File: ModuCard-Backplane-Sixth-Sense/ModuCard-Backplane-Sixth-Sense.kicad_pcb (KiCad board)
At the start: 2 copper layers, 90 parts, among them J16 09031967921, J17 09031967921, J18 09031967921, J19 09031967921, J2 09031967921, J20 09031967921, J21 09031967921, J4 09031967921, SW1 SW_DIP_x02, SW2 SW_DIP_x02, U3 AMS1117, U4 FE2.1, U801 FSUSB42UMX, U802 FSUSB42UMX, X2 X322512MSB4SI

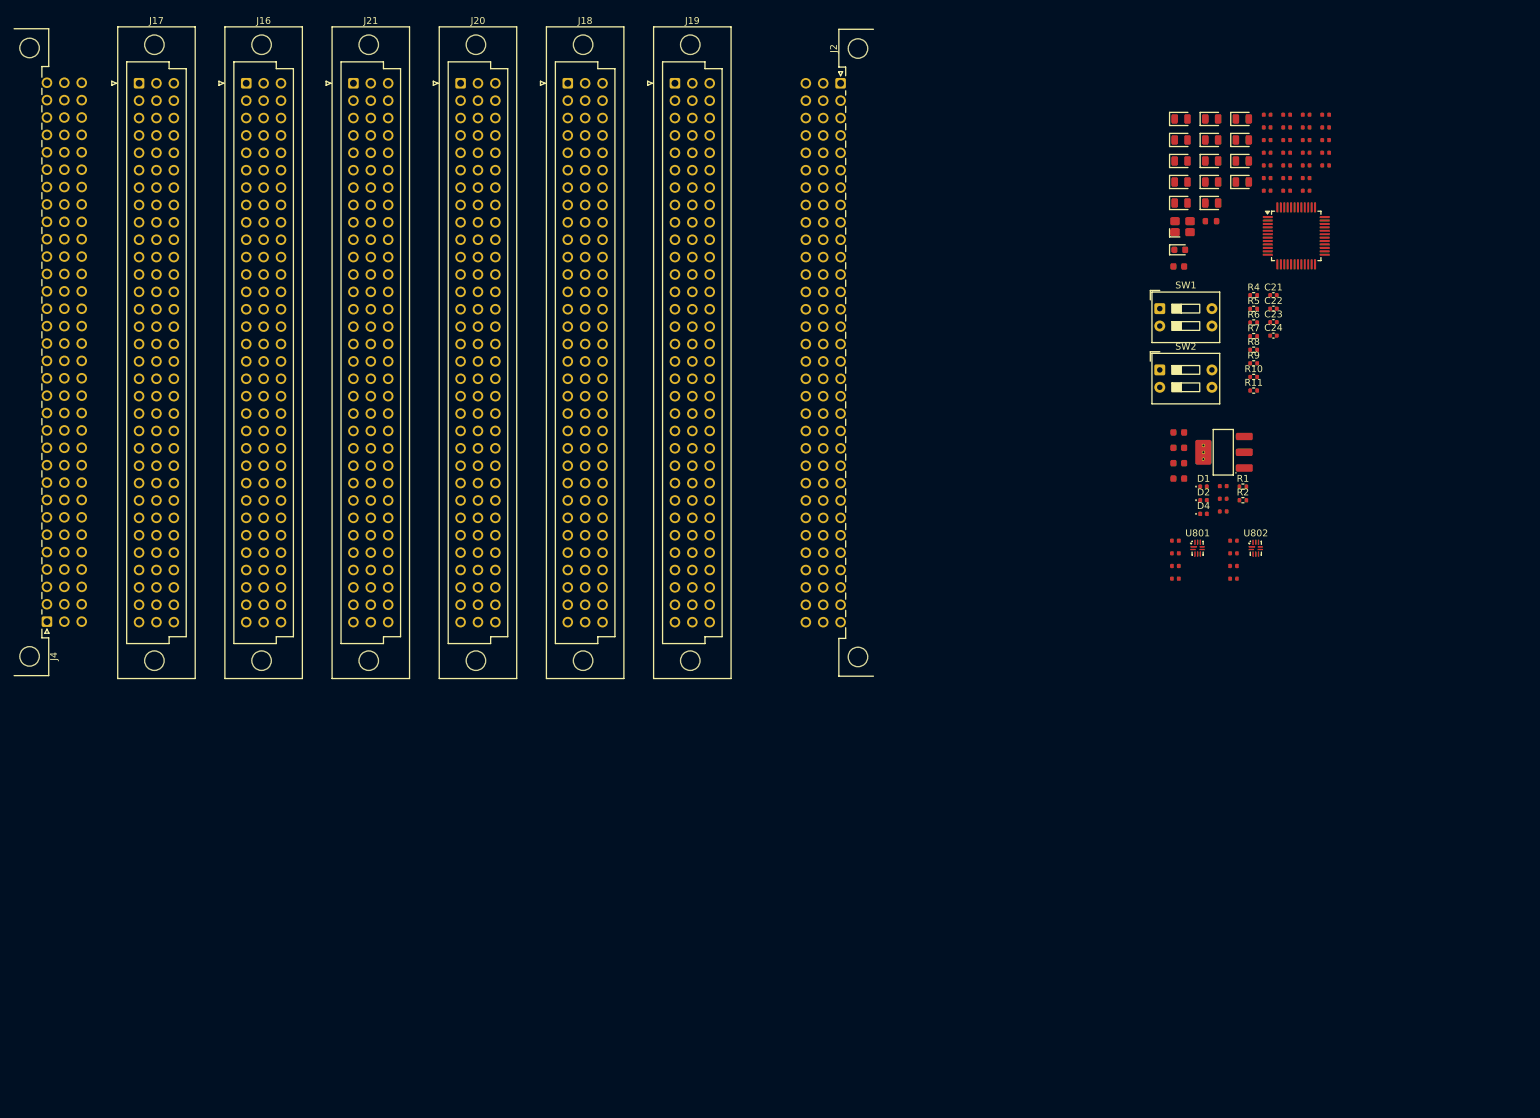
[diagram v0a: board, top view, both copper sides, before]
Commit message: erc -fix1
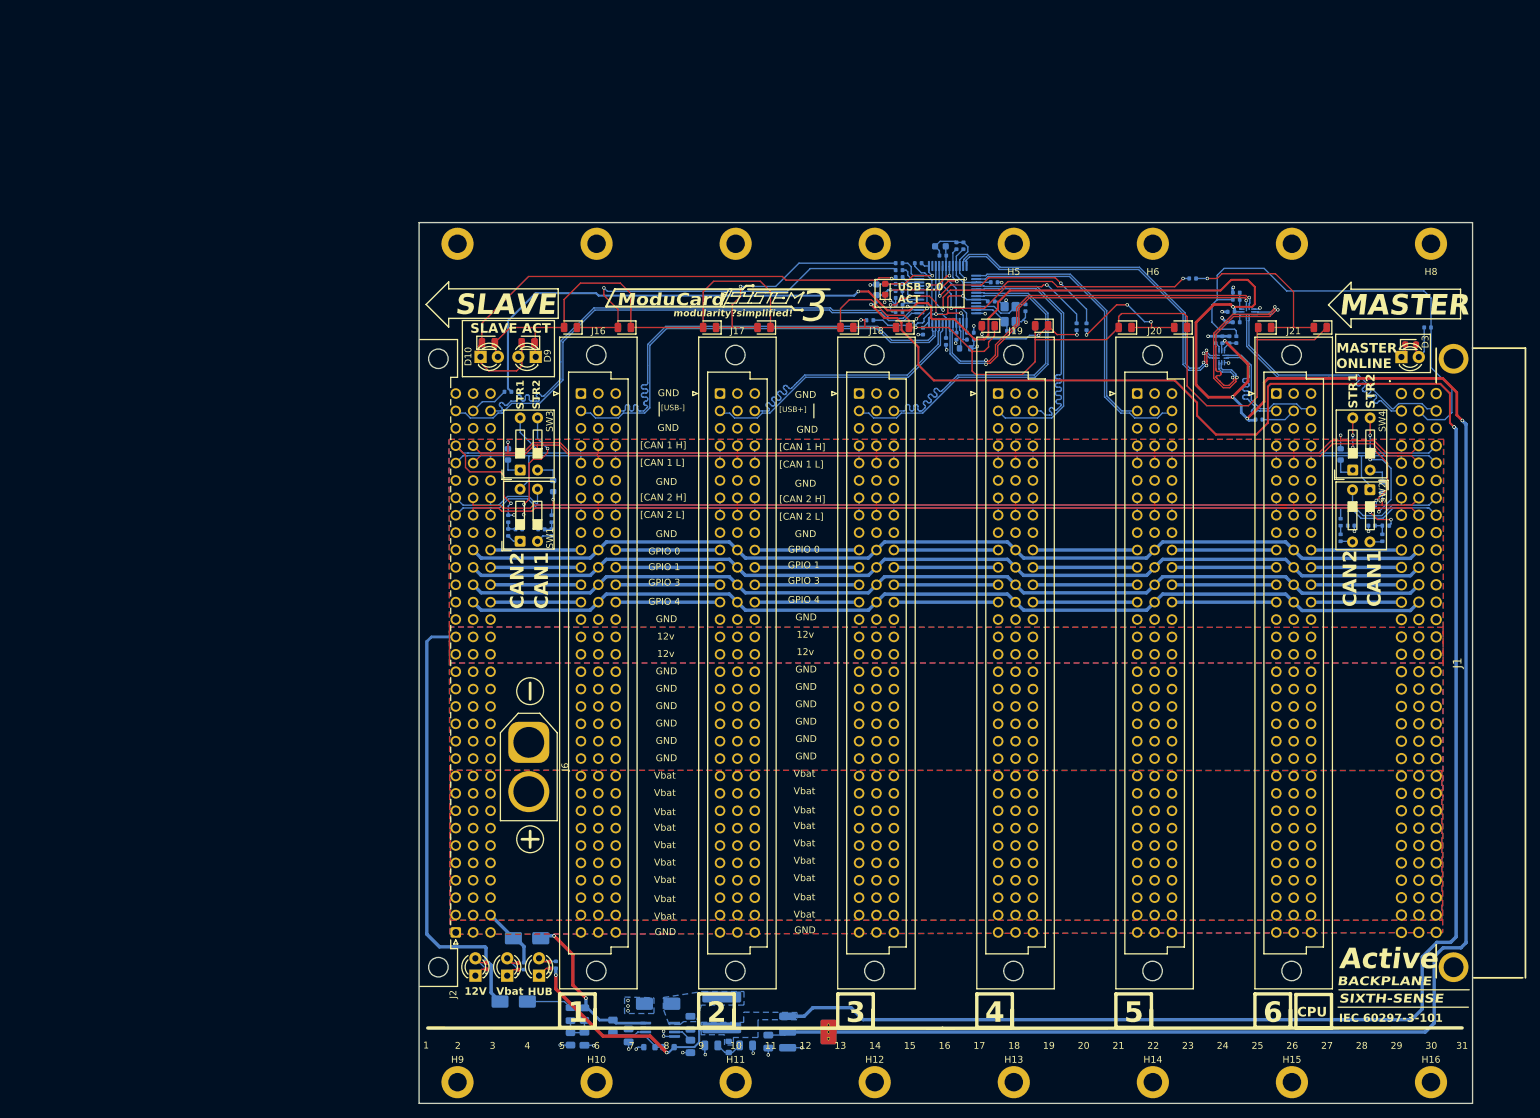
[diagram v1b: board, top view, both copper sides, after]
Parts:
- removed C28: 100nF, PCM_JLCPCB:C_0402
- removed C3, C5: 10uF, PCM_JLCPCB:C_0603
- removed C4, C6: 100nF, PCM_JLCPCB:C_0603
- removed J4: 09031967921, Connector_DIN:DIN41612_R_3x32_Female_Horizontal_THT
- removed R2: 1K2, Resistor_SMD:R_0402_1005Metric
- added C1: 10nF, PCM_JLCPCB:C_0805, B.Cu at (173.2, 200.7)
- added C10: 10uF, PCM_JLCPCB:C_0805, B.Cu at (176.3, 204.0)
- added C11: 10uF, PCM_JLCPCB:C_0805, B.Cu at (184.6, 203.4)
- added C2: 100nF, PCM_JLCPCB:C_0805, B.Cu at (164.2, 202.5)
- added C41: 10uF, PCM_JLCPCB:C_0603, B.Cu at (200.4, 93.5)
- added C7: 10uF, PCM_JLCPCB:C_0805, B.Cu at (155.7, 199.4)
- added C8: 10uF, PCM_JLCPCB:C_0805, B.Cu at (157.7, 203.0)
- added C9: 10uF, PCM_JLCPCB:C_0805, B.Cu at (181.4, 204.0)
- added D10: LED, LED_THT:LED_D3.0mm, F.Cu at (142.6, 103.3)
- added D11: LED, LED_THT:LED_D3.0mm, F.Cu at (141.8, 193.8)
- added D12: LED, LED_THT:LED_D3.0mm, F.Cu at (146.4, 193.8)
- added D13: LED, LED_THT:LED_D3.0mm, F.Cu at (151.1, 193.8)
- added D3: LED, LED_THT:LED_D3.0mm_Clear, F.Cu at (277.1, 103.4)
- added D5: SS510, PCM_JLCPCB:D_SMA, B.Cu at (168.5, 197.9)
- added D6: SS510, PCM_JLCPCB:D_SMA, B.Cu at (149.3, 188.3)
- added D7: SS510, PCM_JLCPCB:D_SMA, B.Cu at (147.4, 197.6)
- added D8: RED, Diode_SMD:D_0402_1005Metric, F.Cu at (152.7, 192.2)
- added D9: LED, LED_THT:LED_D3.0mm, F.Cu at (150.6, 103.3)
- added G***: LOGO, LOGO, B.Cu at (264.6, 200.7)
- added G***: LOGO, LOGO, B.Cu at (246.2, 200.5)
- added H1: MountingHole, MountingHole:MountingHole_2.7mm_M2.5_DIN965_Pad, F.Cu at (139.2, 86.8)
- added H10: MountingHole, MountingHole:MountingHole_2.7mm_M2.5_DIN965_Pad, F.Cu at (159.5, 209.3)
- added H11: MountingHole, MountingHole:MountingHole_2.7mm_M2.5_DIN965_Pad, F.Cu at (179.8, 209.3)
- added H12: MountingHole, MountingHole:MountingHole_2.7mm_M2.5_DIN965_Pad, F.Cu at (200.1, 209.3)
- added H13: MountingHole, MountingHole:MountingHole_2.7mm_M2.5_DIN965_Pad, F.Cu at (220.5, 209.3)
- added H14: MountingHole, MountingHole:MountingHole_2.7mm_M2.5_DIN965_Pad, F.Cu at (240.8, 209.3)
- added H15: MountingHole, MountingHole:MountingHole_2.7mm_M2.5_DIN965_Pad, F.Cu at (261.1, 209.3)
- added H16: MountingHole, MountingHole:MountingHole_2.7mm_M2.5_DIN965_Pad, F.Cu at (281.4, 209.3)
- added H2: MountingHole, MountingHole:MountingHole_2.7mm_M2.5_DIN965_Pad, F.Cu at (159.5, 86.8)
- added H3: MountingHole, MountingHole:MountingHole_2.7mm_M2.5_DIN965_Pad, F.Cu at (179.8, 86.8)
- added H4: MountingHole, MountingHole:MountingHole_2.7mm_M2.5_DIN965_Pad, F.Cu at (200.1, 86.8)
- added H5: MountingHole, MountingHole:MountingHole_2.7mm_M2.5_DIN965_Pad, F.Cu at (220.5, 86.8)
- added H6: MountingHole, MountingHole:MountingHole_2.7mm_M2.5_DIN965_Pad, F.Cu at (240.8, 86.8)
- added H7: MountingHole, MountingHole:MountingHole_2.7mm_M2.5_DIN965_Pad, F.Cu at (261.1, 86.8)
- added H8: MountingHole, MountingHole:MountingHole_2.7mm_M2.5_DIN965_Pad, F.Cu at (281.4, 86.8)
- added H9: MountingHole, MountingHole:MountingHole_2.7mm_M2.5_DIN965_Pad, F.Cu at (139.2, 209.3)
- added J1: 09031967921, Din:09031967921, F.Cu at (282.2, 108.7)
- added J6: Conn_01x02_Pin, Connector_AMASS:AMASS_XT60-F_1x02_P7.20mm_Vertical, F.Cu at (149.6, 159.7)
- added L1: FNR6045S101MT 100uH, Inductor_SMD:L_Chilisin_BWVS00606020, B.Cu at (177.8, 199.1)
- added R12: 100kΩ, PCM_JLCPCB:R_0805, B.Cu at (173.2, 204.1)
- added R13: 3kΩ, PCM_JLCPCB:R_0603, B.Cu at (170.0, 204.2)
- added R14: 3kΩ, PCM_JLCPCB:R_0603, B.Cu at (167.2, 204.2)
- added R15: 100kΩ, PCM_JLCPCB:R_0805, B.Cu at (157.7, 199.4)
- added R16: 100kΩ, PCM_JLCPCB:R_0805, B.Cu at (155.7, 203.0)
- added R17: 1Ω, PCM_JLCPCB:R_0603, B.Cu at (178.8, 204.2)
- added R18: 1K2, Resistor_SMD:R_0402_1005Metric, B.Cu at (153.6, 192.2)
- added R21: 100Ω, PCM_JLCPCB:R_0603, B.Cu at (146.6, 117.6)
- added R22: 100Ω, PCM_JLCPCB:R_0603, B.Cu at (153.2, 122.2)
- added R23: 100Ω, PCM_JLCPCB:R_0603, B.Cu at (268.2, 117.6)
- added R24: 100Ω, PCM_JLCPCB:R_0603, B.Cu at (274.3, 122.4)
- added R3: 200kΩ, PCM_JLCPCB:R_0805, B.Cu at (161.9, 201.2)
- added R39: 330Ω, PCM_JLCPCB:R_0402, B.Cu at (280.9, 99.1)
- added SW3: SW_DIP_x02, Button_Switch_THT:SW_DIP_SPSTx02_Slide_9.78x7.26mm_W7.62mm_P2.54mm, F.Cu at (148.3, 119.9)
- added SW4: SW_DIP_x02, Button_Switch_THT:SW_DIP_SPSTx02_Slide_9.78x7.26mm_W7.62mm_P2.54mm, F.Cu at (270.0, 119.9)
- added U1: LM5007MM, Package_SO:MSOP-8_3x3mm_P0.65mm, B.Cu at (168.8, 201.7)
- C21, C22, C23, C24, C25, C26, C27, C29, C30, C31, C312, C313, C32, C33, C34, C35, C36, C37, C38, C39, C40, R1, R10, R11, R19, R25, R26, R27, R28, R29, R30, R31, R32, R33, R34, R35, R36, R37, R38, R4, R5, R6, R7, R8, R802, R803, R804, R805, R806, R807, R9, U3, U4, U801, U802, X2: moved to B.Cu
- D2: value RED -> Red; footprint Diode_SMD:D_0402_1005Metric -> PCM_JLCPCB:D_0603
- J2: footprint Connector_DIN:DIN41612_R_3x32_Female_Horizontal_THT -> Connector_DIN:DIN41612_R_3x32_Male_Horizontal_THT
- moved J21 142.3 mm to (258.8, 108.7)
- moved J2 136.2 mm to (138.9, 187.5), turned to 90 degrees
- moved R19 128.5 mm to (143.3, 192.3), turned to 90 degrees
- moved R1 126.3 mm to (148.9, 192.4), turned to -90 degrees
- moved D4 123.9 mm to (143.3, 192.3), turned to 90 degrees
- moved D1 122.3 mm to (148.0, 192.4), turned to 90 degrees
- moved C21 115.4 mm to (148.2, 128.6)
- moved R5 113.7 mm to (146.6, 129.0), turned to 90 degrees
- moved R4 113.7 mm to (146.6, 127.0), turned to 90 degrees
- moved D33 112.6 mm to (143.7, 101.3)
- moved C23 111.2 mm to (151.4, 128.6), turned to 180 degrees
- moved J20 108.8 mm to (238.5, 108.7)
- moved D32 107.7 mm to (149.5, 101.3), turned to 180 degrees
- moved R26 106.0 mm to (146.6, 108.5)
- moved R9 105.5 mm to (152.9, 129.0), turned to 90 degrees
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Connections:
- C27 pad 1: /FE2.1/VDD5 -> +5V
- D20 pad 2: Net-(D20-Pad2) -> Net-(D10-A)
- D21 pad 1: Net-(D20-Pad2) -> Net-(D10-A)
- D22 pad 2: Net-(D20-Pad2) -> Net-(D10-A)
- D23 pad 1: Net-(D20-Pad2) -> Net-(D10-A)
- D24 pad 2: Net-(D20-Pad2) -> Net-(D10-A)
- D25 pad 1: Net-(D20-Pad2) -> Net-(D10-A)
- D26 pad 2: Net-(D20-Pad2) -> Net-(D10-A)
- D27 pad 1: Net-(D20-Pad2) -> Net-(D10-A)
- D28 pad 2: Net-(D20-Pad2) -> Net-(D10-A)
- D29 pad 1: Net-(D20-Pad2) -> Net-(D10-A)
- D30 pad 2: Net-(D20-Pad2) -> Net-(D10-A)
- D31 pad 1: Net-(D20-Pad2) -> Net-(D10-A)
- D32 pad 1: Net-(D32-Pad1) -> Net-(D10-A)
- D32 pad 2: Net-(D20-Pad2) -> Net-(D10-K)
- D33 pad 1: Net-(D20-Pad2) -> Net-(D10-K)
- D33 pad 2: Net-(D32-Pad1) -> Net-(D10-A)
- J16 pad a10: /Ext-Connector2/GPIOR0 -> /Ext-Connector/GPIOR0
- J16 pad a11: /Ext-Connector2/GPIOR1 -> /Ext-Connector/GPIOR1
- J16 pad a12: /Ext-Connector2/GPIOR2 -> /Ext-Connector/GPIOR2
- J16 pad a13: /Ext-Connector2/GPIOR3 -> /Ext-Connector/GPIOR3
- J16 pad b4: /Can Split Terminators/CAN1.+ -> /Can Split Terminators/Strobe1.+
- J16 pad b5: /Can Split Terminators/CAN1.- -> /Can Split Terminators/Strobe1.-
- J16 pad b7: /Can Split Terminators/CAN2.+ -> /Can Split Terminators/Strobe2.+
- J16 pad b8: /Can Split Terminators/CAN2.- -> /Can Split Terminators/Strobe2.-
- J17 pad b4: /Can Split Terminators/CAN1.+ -> /Can Split Terminators/Strobe1.+
- J17 pad b5: /Can Split Terminators/CAN1.- -> /Can Split Terminators/Strobe1.-
- J17 pad b7: /Can Split Terminators/CAN2.+ -> /Can Split Terminators/Strobe2.+
- J17 pad b8: /Can Split Terminators/CAN2.- -> /Can Split Terminators/Strobe2.-
- J18 pad a2: /FE2.1/USB4.D- -> /FE2.1/USB1.D-
- J18 pad b4: /Can Split Terminators/CAN1.+ -> /Can Split Terminators/Strobe1.+
- J18 pad b5: /Can Split Terminators/CAN1.- -> /Can Split Terminators/Strobe1.-
- J18 pad b7: /Can Split Terminators/CAN2.+ -> /Can Split Terminators/Strobe2.+
- J18 pad b8: /Can Split Terminators/CAN2.- -> /Can Split Terminators/Strobe2.-
- J18 pad c2: /FE2.1/USB4.D+ -> /FE2.1/USB1.D+
- J19 pad a2: /FE2.1/USB3.D- -> /FE2.1/USB2.D-
- J19 pad b4: /Can Split Terminators/CAN1.+ -> /Can Split Terminators/Strobe1.+
- J19 pad b5: /Can Split Terminators/CAN1.- -> /Can Split Terminators/Strobe1.-
- J19 pad b7: /Can Split Terminators/CAN2.+ -> /Can Split Terminators/Strobe2.+
- J19 pad b8: /Can Split Terminators/CAN2.- -> /Can Split Terminators/Strobe2.-
- J19 pad c2: /FE2.1/USB3.D+ -> /FE2.1/USB2.D+
- J2 pad a10: /Ext-Connector/GPIOL0 -> Vbat
- J2 pad a11: /Ext-Connector/GPIOL1 -> GND
- J2 pad a12: /Ext-Connector/GPIOL2 -> GND
- J2 pad a13: /Ext-Connector/GPIOL3 -> GND
- J2 pad a15: +12V -> GND
- J2 pad a16: +12V -> GND
- J2 pad a17: GND -> +12V
- J2 pad a18: GND -> +12V
- J2 pad a2: /Ext-Connector/USB.D- -> Vbat
- J2 pad a20: GND -> /Ext-Connector/GPIOL3
- J2 pad a21: GND -> /Ext-Connector/GPIOL2
- J2 pad a22: GND -> /Ext-Connector/GPIOL1
- J2 pad a23: Vbat -> /Ext-Connector/GPIOL0
- J2 pad a24: Vbat -> GND
- J2 pad a25: Vbat -> /Can Split Terminators/CAN2.-
- J2 pad a26: Vbat -> /Can Split Terminators/CAN2.+
- J2 pad a27: Vbat -> GND
- J2 pad a28: Vbat -> /Can Split Terminators/CAN1.-
- J2 pad a29: Vbat -> /Can Split Terminators/CAN1.+
- J2 pad a3: GND -> Vbat
- J2 pad a30: Vbat -> GND
- J2 pad a31: Vbat -> /Ext-Connector/USB.D-
- J2 pad a4: /Can Split Terminators/CAN1.+ -> Vbat
- J2 pad a5: /Can Split Terminators/CAN1.- -> Vbat
- J2 pad a6: GND -> Vbat
- J2 pad a7: /Can Split Terminators/CAN2.+ -> Vbat
- J2 pad a8: /Can Split Terminators/CAN2.- -> Vbat
- J2 pad a9: GND -> Vbat
- J2 pad b10: /Ext-Connector/GPIOC0 -> Vbat
- J2 pad b11: /Ext-Connector/GPIOC1 -> GND
- J2 pad b12: /Ext-Connector/GPIOC2 -> GND
- J2 pad b13: /Ext-Connector/GPIOC3 -> GND
- J2 pad b15: +12V -> GND
- J2 pad b16: +12V -> GND
- J2 pad b17: GND -> +12V
- J2 pad b18: GND -> +12V
- J2 pad b2: /Ext-Connector/Index -> Vbat
- J2 pad b20: GND -> /Ext-Connector/GPIOC3
- J2 pad b21: GND -> /Ext-Connector/GPIOC2
- J2 pad b22: GND -> /Ext-Connector/GPIOC1
- J2 pad b23: Vbat -> /Ext-Connector/GPIOC0
- J2 pad b24: Vbat -> GND
- J2 pad b25: Vbat -> /Can Split Terminators/Strobe2.-
- J2 pad b26: Vbat -> /Can Split Terminators/Strobe2.+
- J2 pad b27: Vbat -> GND
- J2 pad b28: Vbat -> /Can Split Terminators/Strobe1.-
- J2 pad b29: Vbat -> /Can Split Terminators/Strobe1.+
- J2 pad b3: GND -> Vbat
- J2 pad b30: Vbat -> GND
- J2 pad b31: Vbat -> /Ext-Connector/Index
- J2 pad b4: /Can Split Terminators/CAN1.+ -> Vbat
- J2 pad b5: /Can Split Terminators/CAN1.- -> Vbat
- J2 pad b6: GND -> Vbat
- J2 pad b7: /Can Split Terminators/CAN2.+ -> Vbat
- J2 pad b8: /Can Split Terminators/CAN2.- -> Vbat
- J2 pad b9: GND -> Vbat
- J2 pad c10: /Ext-Connector/GPIOR0 -> Vbat
- J2 pad c11: /Ext-Connector/GPIOR1 -> GND
- J2 pad c12: /Ext-Connector/GPIOR2 -> GND
- J2 pad c13: /Ext-Connector/GPIOR3 -> GND
- J2 pad c15: +12V -> GND
- J2 pad c16: +12V -> GND
- J2 pad c17: GND -> +12V
- J2 pad c18: GND -> +12V
- J2 pad c2: /Ext-Connector/USB.D+ -> Vbat
- J2 pad c20: GND -> /Ext-Connector/GPIOR3
- J2 pad c21: GND -> /Ext-Connector/GPIOR2
- J2 pad c22: GND -> /Ext-Connector/GPIOR1
- J2 pad c23: Vbat -> /Ext-Connector/GPIOR0
- J2 pad c24: Vbat -> GND
- J2 pad c25: Vbat -> /Can Split Terminators/CAN2.-
- J2 pad c26: Vbat -> /Can Split Terminators/CAN2.+
- J2 pad c27: Vbat -> GND
- J2 pad c28: Vbat -> /Can Split Terminators/CAN1.-
- J2 pad c29: Vbat -> /Can Split Terminators/CAN1.+
- J2 pad c3: GND -> Vbat
- J2 pad c30: Vbat -> GND
- J2 pad c31: Vbat -> /Ext-Connector/USB.D+
- J2 pad c4: /Can Split Terminators/CAN1.+ -> Vbat
- J2 pad c5: /Can Split Terminators/CAN1.- -> Vbat
- J2 pad c6: GND -> Vbat
- J2 pad c7: /Can Split Terminators/CAN2.+ -> Vbat
- J2 pad c8: /Can Split Terminators/CAN2.- -> Vbat
- J2 pad c9: GND -> Vbat
- J20 pad a2: /FE2.1/USB2.D- -> /FE2.1/USB3.D-
- J20 pad b4: /Can Split Terminators/CAN1.+ -> /Can Split Terminators/Strobe1.+
- J20 pad b5: /Can Split Terminators/CAN1.- -> /Can Split Terminators/Strobe1.-
- J20 pad b7: /Can Split Terminators/CAN2.+ -> /Can Split Terminators/Strobe2.+
- J20 pad b8: /Can Split Terminators/CAN2.- -> /Can Split Terminators/Strobe2.-
- J20 pad c2: /FE2.1/USB2.D+ -> /FE2.1/USB3.D+
- J21 pad b4: /Can Split Terminators/CAN1.+ -> /Can Split Terminators/Strobe1.+
- J21 pad b5: /Can Split Terminators/CAN1.- -> /Can Split Terminators/Strobe1.-
- J21 pad b7: /Can Split Terminators/CAN2.+ -> /Can Split Terminators/Strobe2.+
- J21 pad b8: /Can Split Terminators/CAN2.- -> /Can Split Terminators/Strobe2.-
- J21 pad c10: /Ext-Connector/GPIOL0 -> /Ext-conn-M/GPIOR0
- J21 pad c11: /Ext-Connector/GPIOL1 -> /Ext-conn-M/GPIOR1
- J21 pad c12: /Ext-Connector/GPIOL2 -> /Ext-conn-M/GPIOR2
- J21 pad c13: /Ext-Connector/GPIOL3 -> /Ext-conn-M/GPIOR3
- R1 pad 1: unconnected-(R1-Pad1) -> Vbat
- R19 pad 2: +3V3 -> +12V
- R26 pad 1: /Ext-Connector2/Index -> /Ext-Connector/Index
- R28 pad 1: /FE2.1/VDD5 -> +5V
- R37 pad 2: Net-(D32-Pad1) -> Net-(D10-K)
- R38 pad 1: Net-(D20-Pad2) -> Net-(D10-A)
- R802 pad 1: /Ext-Connector/Index -> /Ext-conn-M/Index
- R805 pad 1: /Ext-Connector/Index -> /Ext-conn-M/Index
- U3 pad 3: +5v stdby -> +5V
- U4 pad 37: /Ext-Connector2/USB.D- -> /Ext-Connector/USB.D-
- U4 pad 38: /Ext-Connector2/USB.D+ -> /Ext-Connector/USB.D+
- U4 pad 8: /FE2.1/VDD5 -> +5V
- U4 pad 9: /FE2.1/VD33_O -> /FE2.1/VD33
- U801 pad 6: /Ext-Connector/USB.D- -> /Ext-conn-M/USB.D-
- U801 pad 7: /Ext-Connector/USB.D+ -> /Ext-conn-M/USB.D+
- U802 pad 6: /FE2.1/USB1.D- -> /FE2.1/USB4.D-
- U802 pad 7: /FE2.1/USB1.D+ -> /FE2.1/USB4.D+
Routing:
- net +3V3: track 0.00 -> 409.6 mm, vias 0 -> 6
- net +5V: track 0.00 -> 344.9 mm, vias 0 -> 6
- net Net-(D10-A): track 0.00 -> 212.7 mm, vias 0 -> 1
- net /Can Split Terminators/CAN1.+: track 0.00 -> 192.1 mm, vias 0 -> 6
- net /Can Split Terminators/Strobe2.-: track 0.00 -> 182.0 mm, vias 0 -> 7
- net /Can Split Terminators/CAN1.-: track 0.00 -> 170.0 mm
- net /Can Split Terminators/CAN2.+: track 0.00 -> 166.0 mm
- net /Can Split Terminators/CAN2.-: track 0.00 -> 164.4 mm
- net /Can Split Terminators/Strobe1.-: track 0.00 -> 159.3 mm, vias 0 -> 3
- net /Can Split Terminators/Strobe1.+: track 0.00 -> 153.3 mm, vias 0 -> 2
- net /Can Split Terminators/Strobe2.+: track 0.00 -> 151.0 mm, vias 0 -> 2
- net /Ext-Connector/GPIOC1: track 0.00 -> 145.0 mm
- net /Ext-Connector/GPIOC0: track 0.00 -> 145.0 mm
- net /Ext-Connector/GPIOC2: track 0.00 -> 145.0 mm
- net /Ext-Connector/GPIOC3: track 0.00 -> 145.0 mm
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- added copper zone on B.Cu, net +12V
- added copper zone on F.Cu, net +12V
- added copper zone on In1.Cu, net +12V
- added copper zone on In2.Cu, net +12V
- added copper zone on B.Cu, net +5V
- added copper zone on B.Cu, net GND
- added copper zone on F.Cu, net GND
- added copper zone on In1.Cu, net GND
- added copper zone on In2.Cu, net GND
- added copper zone on B.Cu, net Net-(U1-SW)
- added copper zone on B.Cu, net Vbat
- added copper zone on F.Cu, net Vbat
- added copper zone on In1.Cu, net Vbat
- added copper zone on In2.Cu, net Vbat
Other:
- board outline added: 153.9 x 128.7 mm
- copper layers 2 -> 4
- board text added: "1"
- board text added: "10"
- board text added: "11"
- board text added: "12"
- board text added: "12V"
- board text added: "12v"
- board text added: "13"
- board text added: "14"
- board text added: "15"
- board text added: "16"
- board text added: "17"
- board text added: "18"
- board text added: "19"
- board text added: "2"
- board text added: "20"
- board text added: "21"
- board text added: "22"
- board text added: "23"
- board text added: "24"
- board text added: "25"
- board text added: "26"
- board text added: "27"
- board text added: "28"
- board text added: "29"
- board text added: "3"
- board text added: "30"
- board text added: "31"
- board text added: "4"
- board text added: "5"
- board text added: "6"
- board text added: "7"
- board text added: "8"
- board text added: "9"
- board text added: "Active"
- board text added: "BACKPLANE"
- board text added: "CAN1"
- board text added: "CAN2"
- board text added: "CPU"
- board text added: "DESIGNED IN POLAND"
- board text added: "GND"
- board text added: "GPIO 0"
- board text added: "GPIO 1"
- board text added: "GPIO 3"
- board text added: "GPIO 4"
- board text added: "HUB"
- board text added: "IEC 60297-3-101"
- board text added: "M2.5x10 ISO 14583 TX8"
- board text added: "MASTER"
- board text added: "MASTER ONLINE"
- board text added: "MODULAR MECHANICA Backplane 6-th sense ARTEM.H. :) 2026"
- board text added: "ModuCard"
- board text added: "REV"
- board text added: "SIXTH-SENSE"
- board text added: "SLAVE"
- board text added: "SLAVE ACT"
- board text added: "STR1"
- board text added: "STR2"
- board text added: "USB 2.0"
- board text added: "USB 2.0 ACT"
- board text added: "Vbat"
- board text added: "XA1"
- board text added: "[CAN 1 H]"
- board text added: "[CAN 1 L]"
- board text added: "[CAN 2 H]"
- board text added: "[CAN 2 L]"
- board text added: "[USB+]"
- board text added: "[USB-]"
- board text added: "i"
- board text added: "modularity?simplified!"
